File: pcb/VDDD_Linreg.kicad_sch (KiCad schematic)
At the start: 3 parts, among them U3 TLV70220PDBVR

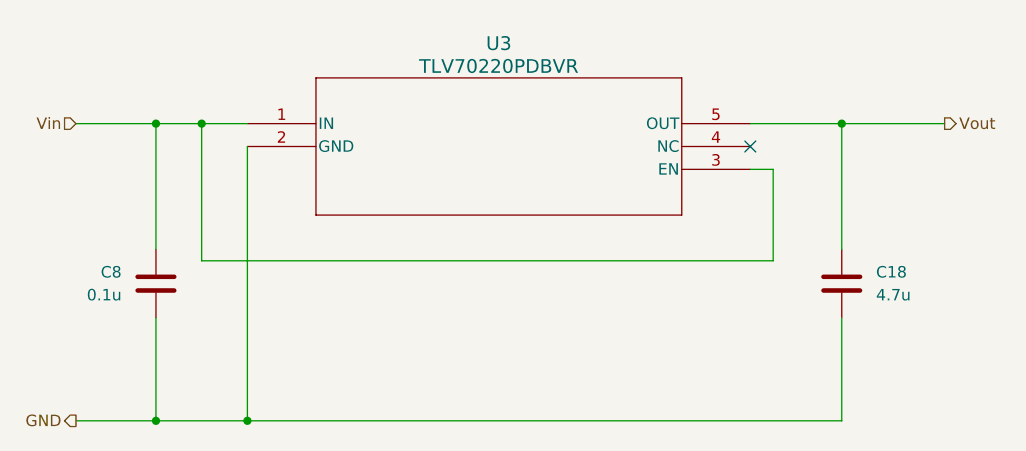
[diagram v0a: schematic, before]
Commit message: Merging in work from FSAE repo from when I forgot this one existed
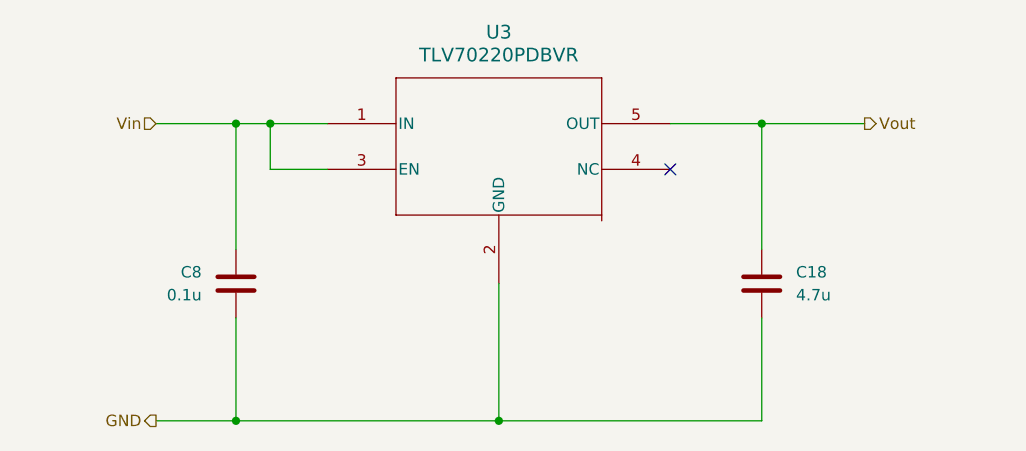
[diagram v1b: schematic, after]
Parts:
- removed U3: TLV70220PDBVR, Package_TO_SOT_SMD:SOT-23-5, symbol ev24:TLV70220PDBVR
- added U3: TLV70220PDBVR, Package_TO_SOT_SMD:SOT-23-5, symbol 0_tlv70220pdbvr:TLV70220PDBVR
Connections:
- net GND: now also U3.2 (GND)
- net Vin: now also U3.1 (IN), U3.3 (EN)
- net Vout: now also U3.5 (OUT)
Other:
- moved on the sheet: C18, C8
